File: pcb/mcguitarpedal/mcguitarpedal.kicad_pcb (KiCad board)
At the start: 2 copper layers, 132.5 x 128 mm, 39 parts, among them J1 IN, J2 PREAMP_HEADERS, J3 BTN_MTX, J4 OUT, J5 EXP, J6 ILI9488 Module, J7 PWR_IN, J8 POTS, SW1 SW_BYPASS, SW2 SW_TUNER, SW3 SW_PRESET, SW4 LINE_LEVEL, U1 Teensy4.0_AudioShield_REVD, U2 Teensy4.1, U3 LM4562, U4 74LS148, U5 HEF4094B, U6 STPDWN-3P-5V, U7 STDN-3A24-ADJ

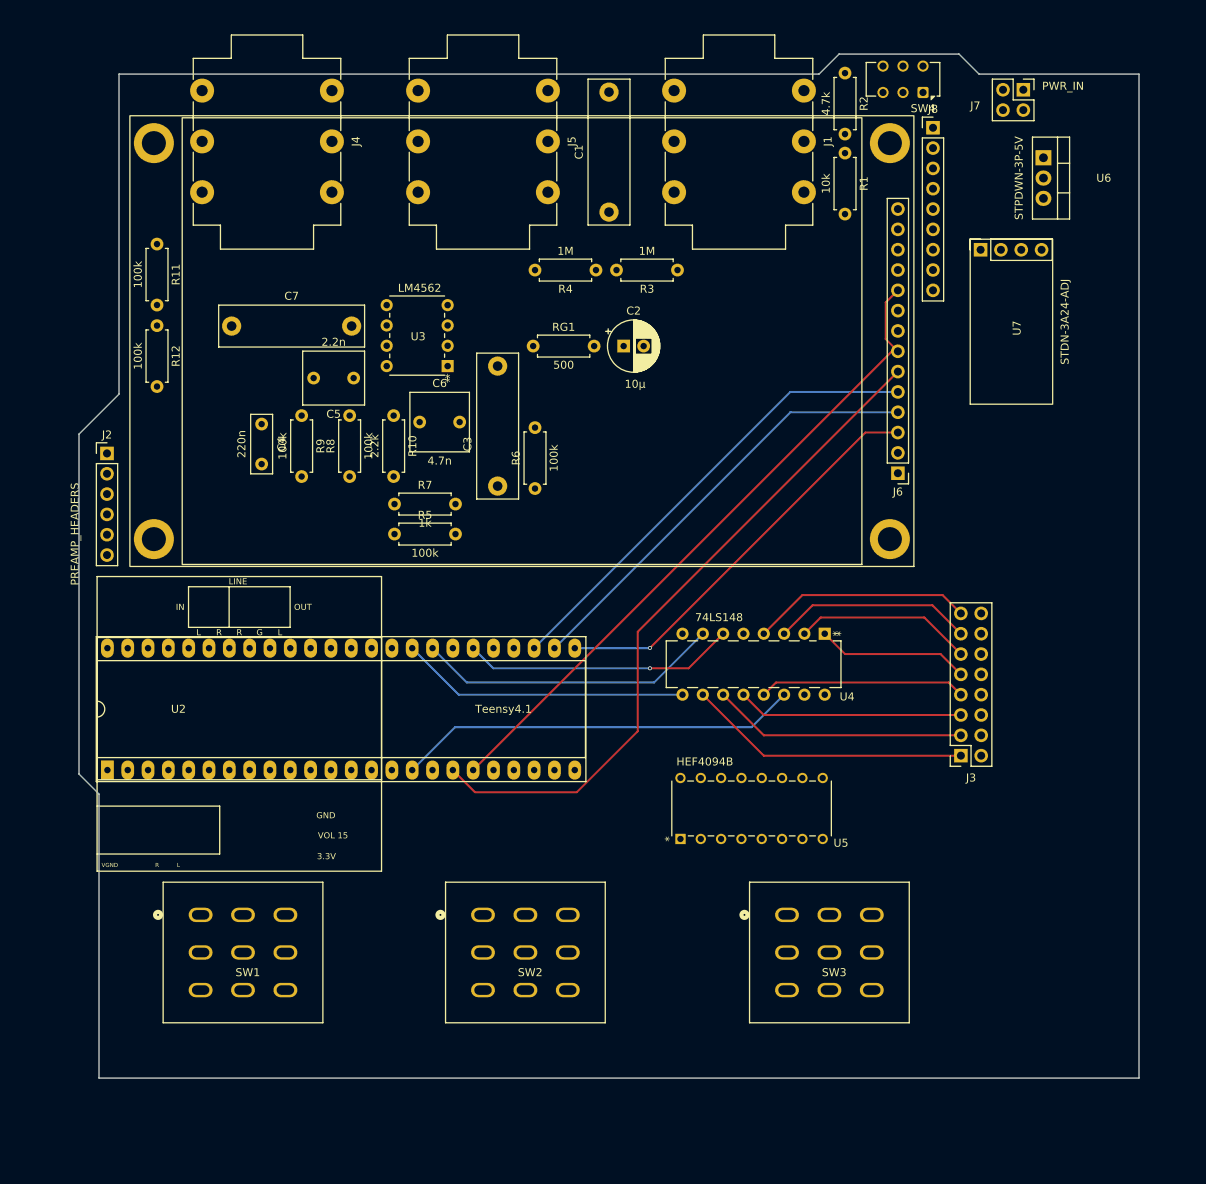
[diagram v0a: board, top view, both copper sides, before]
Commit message: Basic PCB routing
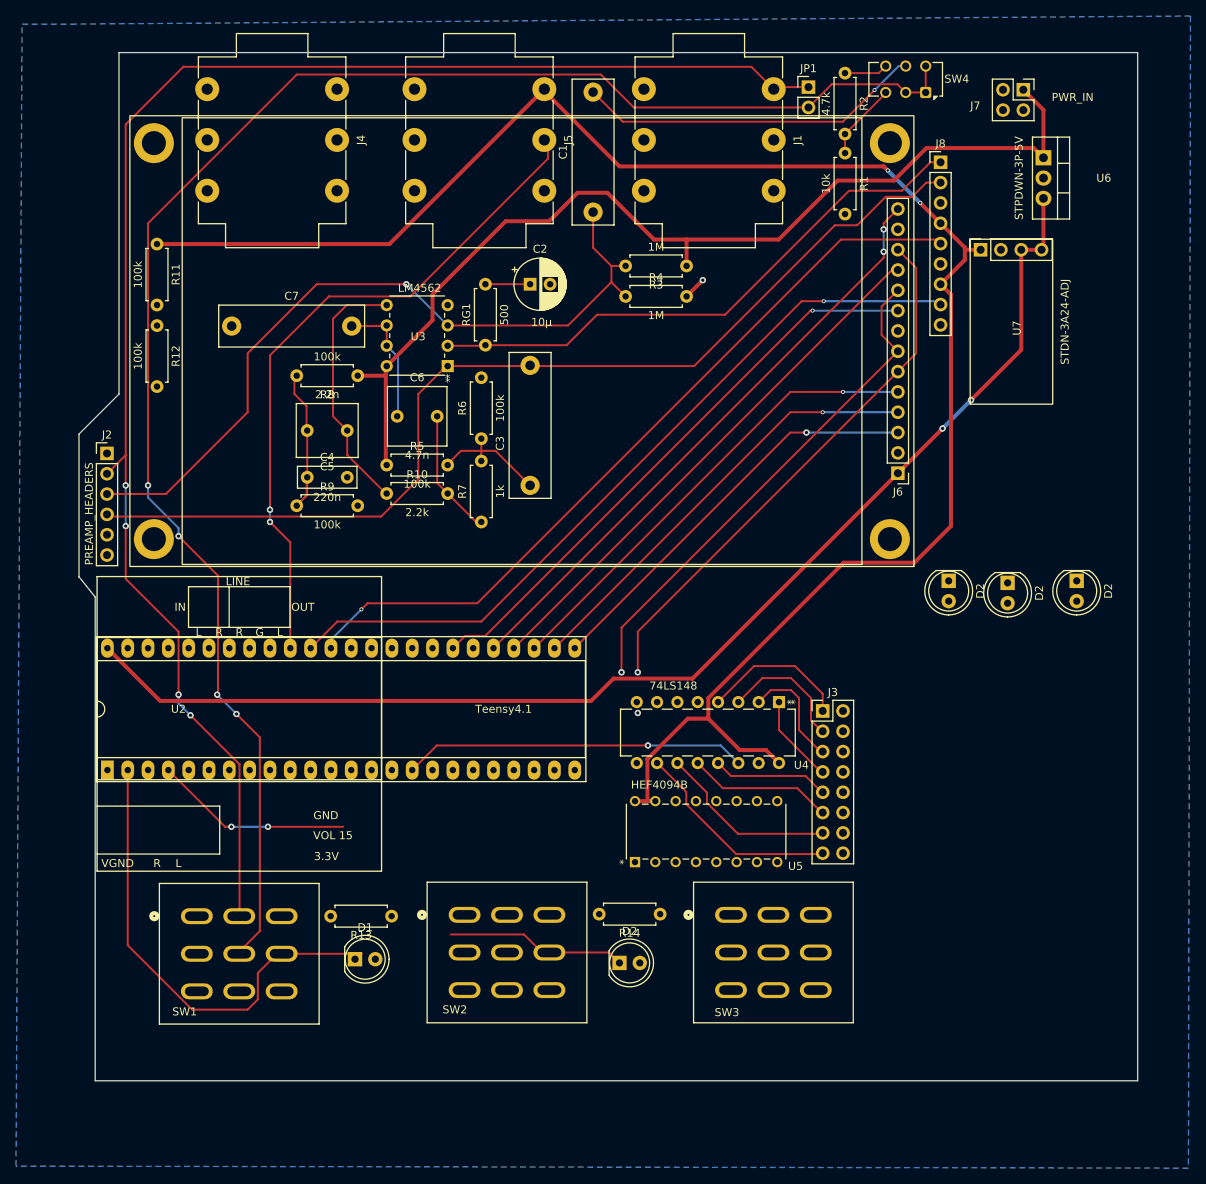
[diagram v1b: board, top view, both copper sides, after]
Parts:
- added D1: LED_BYPASS, LED_THT:LED_D5.0mm, F.Cu at (82.0, 133.1)
- added D2: LED_TUNER, LED_THT:LED_D5.0mm, F.Cu at (163.6, 86.1)
- added D2: LED_TUNER, LED_THT:LED_D5.0mm, F.Cu at (156.2, 85.8)
- added D2: LED_TUNER, LED_THT:LED_D5.0mm, F.Cu at (115.1, 133.6)
- added D2: LED_TUNER, LED_THT:LED_D5.0mm, F.Cu at (172.2, 85.8)
- added JP1: JP_SIGNAL_PREAMP, Connector_PinHeader_2.54mm:PinHeader_1x02_P2.54mm_Vertical, F.Cu at (138.7, 24.1)
- added R13: 150, Resistor_THT:R_Axial_DIN0207_L6.3mm_D2.5mm_P7.62mm_Horizontal, F.Cu at (86.6, 127.8)
- added R14: 150, Resistor_THT:R_Axial_DIN0207_L6.3mm_D2.5mm_P7.62mm_Horizontal, F.Cu at (120.1, 127.5)
- J1, J4, J5: footprint Connector_Audio:Jack_6.35mm_Neutrik_NMJ6HCD2_Horizontal -> mcguitarpedal:Jack_6.35mm_Neutrik_NMJ6HCD2_Horizontal_3D_MODEL
- J3: footprint Connector_PinSocket_2.54mm:PinSocket_2x08_P2.54mm_Vertical -> Connector_PinHeader_2.54mm:PinHeader_2x08_P2.54mm_Vertical
- J8: value POTS -> POT_HP_VOLUME_10k
- moved J3 18.2 mm to (140.5, 102.1), turned to 0 degrees
- moved C2 14.0 mm to (103.9, 48.8)
- moved R8 12.7 mm to (82.3, 60.2), turned to 180 degrees
- moved R9 11.3 mm to (74.7, 76.5), turned to 0 degrees
- moved R7 11.1 mm to (97.8, 78.5), turned to 90 degrees
- moved U4 10.3 mm to (135.0, 101.0)
- moved R10 9.78 mm to (86.0, 74.9), turned to 0 degrees
- moved R6 9.16 mm to (97.8, 68.1)
- moved C4 8.75 mm to (76.0, 72.9), turned to 0 degrees
- moved R5 8.68 mm to (86.0, 71.4)
- moved SW3 7.00 mm to (129.0, 127.6)
- moved C5 6.61 mm to (81.0, 67.1)
- moved U5 6.37 mm to (117.0, 121.0)
- moved RG1 5.97 mm to (98.3, 56.4), turned to 90 degrees
- moved R4 4.96 mm to (115.8, 50.3), turned to 0 degrees
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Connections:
- J1 pad T: /preamp/PREAMP_IN -> /SIGNAL_IN
- J2 pad 2: /preamp/PREAMP_IN -> /SIGNAL_IN
- J4 pad R: Net-(U1-LINE_OUT_GND) -> GND
- J4 pad S: Net-(U1-LINE_OUT_GND) -> GND
- J4 pad T: Net-(U1-LINE_OUT_R) -> Net-(J4-PadT)
- SW1 pad 1: unconnected-(SW1-Pad1) -> /SIGNAL_IN
- SW1 pad 2: unconnected-(SW1-Pad2) -> Net-(J4-PadT)
- SW1 pad 3: unconnected-(SW1-Pad3) -> /LINE_OUT
- SW1 pad 4: unconnected-(SW1-Pad4) -> /SIGNAL_IN
- SW1 pad 5: unconnected-(SW1-Pad5) -> /PREAMP_IN
- SW1 pad 6: unconnected-(SW1-Pad6) -> GND
- SW1 pad 7: unconnected-(SW1-Pad7) -> 3.3V
- SW1 pad 8: unconnected-(SW1-Pad8) -> /1_SW1
- SW1 pad 9: unconnected-(SW1-Pad9) -> GND
- SW2 pad 7: unconnected-(SW2-Pad7) -> 3.3V
- SW2 pad 8: unconnected-(SW2-Pad8) -> /2_SW2
- SW2 pad 9: unconnected-(SW2-Pad9) -> GND
- SW4 pad 1: /preamp/PREAMP_IN -> /PREAMP_IN
- SW4 pad 2: /preamp/PREAMP_IN -> /PREAMP_IN
- SW4 pad 6: /preamp/PREAMP_IN -> /PREAMP_IN
- U2 pad 2: Net-(U1-0_RX1_CRX2_CS1) -> /1_SW1
- U2 pad 37: unconnected-(U2-15_A1_RX3_SPDIF_IN-Pad37) -> /A1_VOLUME
- U2 pad 38: unconnected-(U2-16_A2_RX4_SCL1-Pad38) -> /A2_POT
- U2 pad 39: unconnected-(U2-17_A3_TX4_SDA1-Pad39) -> /A3_EXP
- U2 pad 4: Net-(U1-2_OUT2) -> /2_SW2
- U4 pad 1: Net-(J3-Pin_9) -> Net-(J3-Pin_7)
- U4 pad 10: Net-(J3-Pin_1) -> Net-(J3-Pin_15)
- U4 pad 11: Net-(J3-Pin_3) -> Net-(J3-Pin_13)
- U4 pad 12: Net-(J3-Pin_5) -> Net-(J3-Pin_11)
- U4 pad 13: Net-(J3-Pin_7) -> Net-(J3-Pin_9)
- U4 pad 2: Net-(J3-Pin_11) -> Net-(J3-Pin_5)
- U4 pad 3: Net-(J3-Pin_13) -> Net-(J3-Pin_3)
- U4 pad 4: Net-(J3-Pin_15) -> Net-(J3-Pin_1)
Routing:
- net 3.3V: track 0.00 -> 226.0 mm, vias 0 -> 2
- net /PREAMP_IN: track 0.00 -> 210.0 mm, vias 0 -> 4
- net /SIGNAL_IN: track 0.00 -> 197.4 mm, vias 0 -> 4
- net 5V: track 0.00 -> 156.4 mm, vias 0 -> 2
- net 9V: track 0.00 -> 129.2 mm
- net /preamp/STAGE1_OUT: track 0.00 -> 127.1 mm
- net /preamp/STAGE1_IN: track 0.00 -> 96.6 mm, vias 0 -> 1
- net /A1_VOLUME: track 0.00 -> 96.4 mm, vias 0 -> 1
- net /A2_POT: track 0.00 -> 96.3 mm, vias 0 -> 1
- net /A3_EXP: track 0.00 -> 84.7 mm, vias 0 -> 2
- net /37_TFT_T_IRQ: track 0.00 -> 75.8 mm, vias 0 -> 2
- net /39_TFT_MISO: track 0.00 -> 73.1 mm, vias 0 -> 1
- net Net-(J8A-Pin_1): track 0.00 -> 71.0 mm
- net /36_TOUCH_CS: track 0.00 -> 67.6 mm
- net /1_SW1: track 0.00 -> 58.8 mm
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- added copper zone on B.Cu, net GND
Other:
- board size 132.5 x 128 mm -> 132.3 x 128.5 mm

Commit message: Mostly routed board
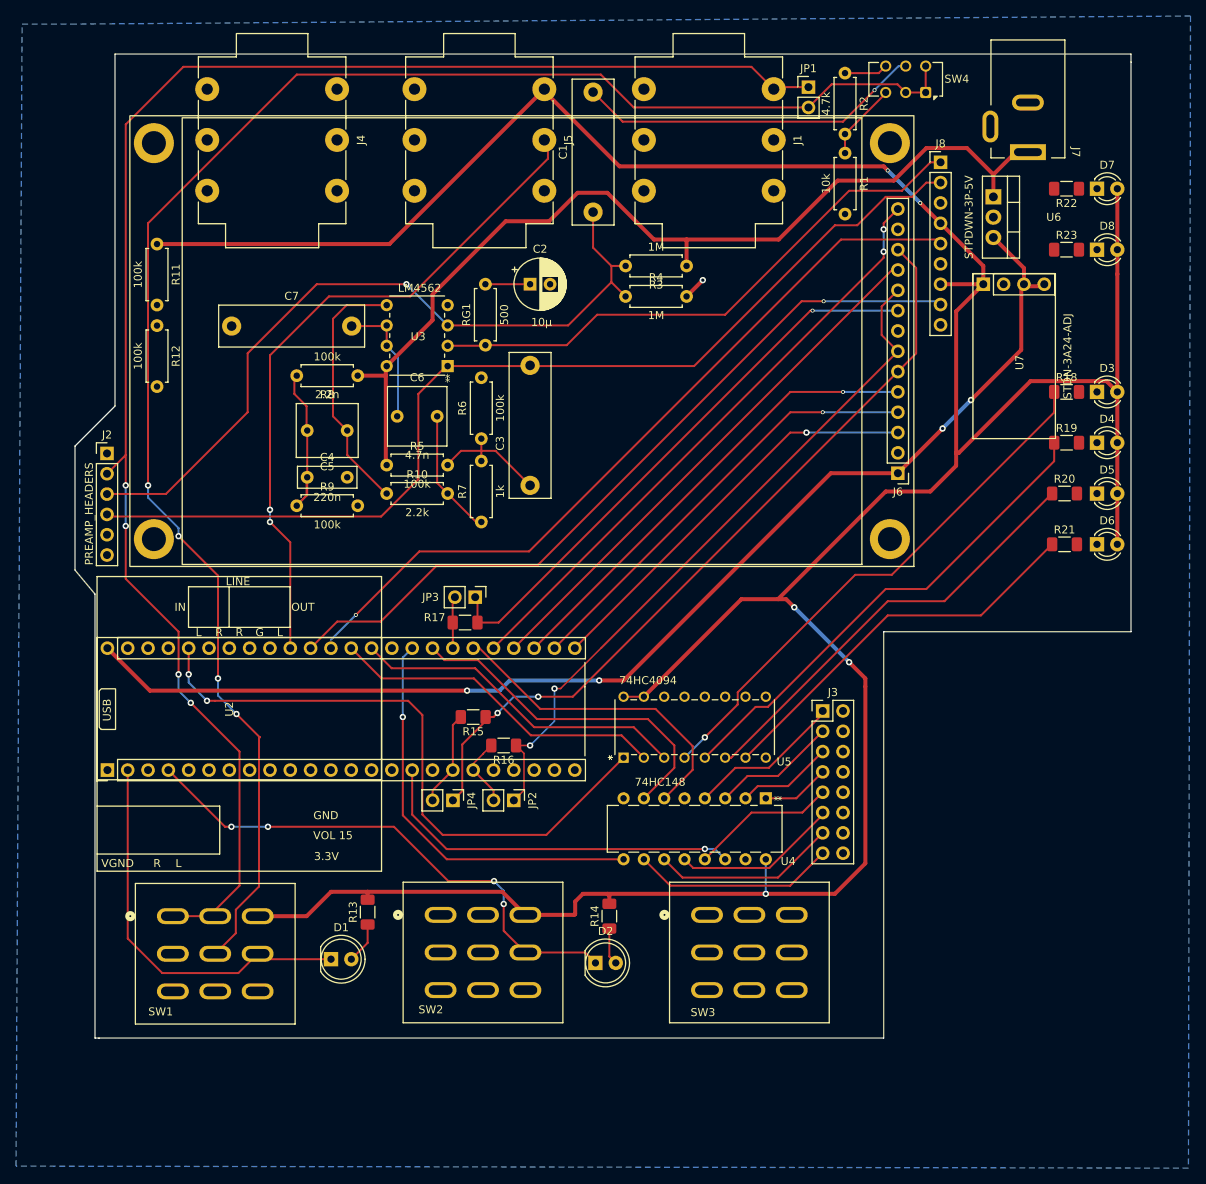
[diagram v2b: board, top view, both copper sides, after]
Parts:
- removed the D2 at (163.6, 86.1)
- removed the D2 at (156.2, 85.8)
- removed the D2 at (172.2, 85.8)
- added D3: LED, LED_THT:LED_D3.0mm, F.Cu at (174.7, 62.2)
- added D4: LED, LED_THT:LED_D3.0mm, F.Cu at (174.7, 68.6)
- added D5: LED, LED_THT:LED_D3.0mm, F.Cu at (174.7, 74.9)
- added D6: LED, LED_THT:LED_D3.0mm, F.Cu at (174.7, 81.3)
- added D7: LED, LED_THT:LED_D3.0mm, F.Cu at (174.8, 36.8)
- added D8: LED, LED_THT:LED_D3.0mm, F.Cu at (174.8, 44.5)
- added JP2: JP_SCLK, Connector_PinHeader_2.54mm:PinHeader_1x02_P2.54mm_Vertical, F.Cu at (101.9, 113.3)
- added JP3: JP_MISO, Connector_PinHeader_2.54mm:PinHeader_1x02_P2.54mm_Vertical, F.Cu at (97.0, 87.9)
- added JP4: JP_MOSI, Connector_PinHeader_2.54mm:PinHeader_1x02_P2.54mm_Vertical, F.Cu at (94.2, 113.3)
- added R15: 50, Resistor_SMD:R_1206_3216Metric_Pad1.30x1.75mm_HandSolder, F.Cu at (96.8, 102.9)
- added R16: 50, Resistor_SMD:R_1206_3216Metric_Pad1.30x1.75mm_HandSolder, F.Cu at (100.6, 106.4)
- added R17: 50, Resistor_SMD:R_1206_3216Metric_Pad1.30x1.75mm_HandSolder, F.Cu at (95.8, 91.1)
- added R18: 150, Resistor_SMD:R_1206_3216Metric_Pad1.30x1.75mm_HandSolder, F.Cu at (170.9, 62.2)
- added R19: 150, Resistor_SMD:R_1206_3216Metric_Pad1.30x1.75mm_HandSolder, F.Cu at (170.9, 68.6)
- added R20: 150, Resistor_SMD:R_1206_3216Metric_Pad1.30x1.75mm_HandSolder, F.Cu at (170.7, 74.9)
- added R21: 150, Resistor_SMD:R_1206_3216Metric_Pad1.30x1.75mm_HandSolder, F.Cu at (170.7, 81.3)
- added R22: 150, Resistor_SMD:R_1206_3216Metric_Pad1.30x1.75mm_HandSolder, F.Cu at (170.9, 36.8)
- added R23: 150, Resistor_SMD:R_1206_3216Metric_Pad1.30x1.75mm_HandSolder, F.Cu at (170.9, 44.5)
- J7: footprint Connector_PinHeader_2.54mm:PinHeader_2x02_P2.54mm_Vertical -> Connector_BarrelJack:BarrelJack_Kycon_KLDX-0202-xC_Horizontal
- R13, R14: footprint Resistor_THT:R_Axial_DIN0207_L6.3mm_D2.5mm_P7.62mm_Horizontal -> Resistor_SMD:R_1206_3216Metric_Pad1.30x1.75mm_HandSolder
- U2: footprint Package_DIP:DIP-48_W15.24mm_Socket_LongPads -> mcguitarpedal:PinHeader_2x24_P2.54mm_W15.24_Vertical
- U4: value 74LS148 -> 74HC148
- U5: value HEF4094B -> 74HC4094
- moved U5 13.1 mm to (115.6, 108.0)
- moved U4 12.1 mm to (133.3, 113.0)
- moved U6 7.94 mm to (161.8, 37.8)
- moved J7 7.82 mm to (166.1, 32.3)
- moved R14 6.36 mm to (113.8, 127.8), turned to 90 degrees
- moved U7 4.32 mm to (160.5, 48.8)
- moved R13 3.04 mm to (83.6, 127.3), turned to 90 degrees
- moved D1 3.00 mm to (79.0, 133.1)
- moved D2 3.00 mm to (112.1, 133.6)
- moved SW1 3.00 mm to (59.2, 127.8)
- moved SW2 3.00 mm to (92.7, 127.6)
- moved SW3 3.00 mm to (126.0, 127.6)
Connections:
- J6 pad 10: /27_TFT_SCLK -> Net-(J6-SCK)
- J6 pad 12: /26_TFT_MOSI -> Net-(J6-SDI(MOSI))
- J6 pad 13: /39_TFT_MISO -> Net-(J6-SDO(MISO))
- J6 pad 6: /26_TFT_MOSI -> Net-(J6-SDI(MOSI))
- J6 pad 7: /27_TFT_SCLK -> Net-(J6-SCK)
- J6 pad 9: /39_TFT_MISO -> Net-(J6-SDO(MISO))
- U5 pad 13: unconnected-(U5-QP5-Pad13) -> Net-(U5-QP5)
- U5 pad 14: unconnected-(U5-QP4-Pad14) -> Net-(U5-QP4)
- U5 pad 4: unconnected-(U5-QP0-Pad4) -> Net-(U5-QP0)
- U5 pad 5: unconnected-(U5-QP1-Pad5) -> Net-(U5-QP1)
- U5 pad 6: unconnected-(U5-QP2-Pad6) -> Net-(U5-QP2)
- U5 pad 7: unconnected-(U5-QP3-Pad7) -> Net-(U5-QP3)
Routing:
- net 3.3V: track 226.0 -> 401.7 mm, vias 2 -> 5
- net Net-(J6-SDI(MOSI)): track 0.00 -> 99.4 mm, vias 0 -> 2
- net Net-(J6-SCK): track 0.00 -> 87.6 mm, vias 0 -> 2
- net /LED_STR: track 0.00 -> 77.8 mm, vias 0 -> 2
- net Net-(J6-SDO(MISO)): track 0.00 -> 72.0 mm, vias 0 -> 1
- net Net-(U5-QP0): track 0.00 -> 67.5 mm, vias 0 -> 1
- net /39_TFT_MISO: track 73.1 -> 6.50 mm, vias 1 -> 0
- net Net-(U5-QP1): track 0.00 -> 61.3 mm
- net /26_TFT_MOSI: track 68.2 -> 12.2 mm, vias 2 -> 0
- net Net-(U5-QP2): track 0.00 -> 54.5 mm
- net /27_TFT_SCLK: track 63.7 -> 9.39 mm, vias 1 -> 0
- net Net-(U2-41_A17): track 0.00 -> 51.3 mm, vias 0 -> 1
- net Net-(U5-QP3): track 0.00 -> 49.4 mm
- net Net-(U2-40_A16): track 0.00 -> 43.5 mm
- net /SCK: track 0.00 -> 42.3 mm
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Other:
- board size 132.3 x 128.5 mm -> 132 x 123 mm
